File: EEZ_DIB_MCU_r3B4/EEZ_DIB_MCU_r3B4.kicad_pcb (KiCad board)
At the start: 4 copper layers, 139.5 x 70 mm, 119 parts, among them IC1 TPD4E001DRLR, IC11 TPS2051BDBVR, IC12 TPS61169DCKR, IC13 TPD4E001DRLR, IC14 TSC2007IPW, IC2 74AUP1G74DC.125, IC3 CD74HC4050PWR, IC5 LD1117ADT33TR, IC8 AT24C256C-SSHL-B, IC9 N.C., J1 5033981892, J2 67803-8020, J3 HR911130A, J4 Conn_01x22_Socket, Q1 N.C., Q2 2N7002, SW1 TL1100CF160Q, SW2 PEC16-2215F-S0024, U1 ICN6211, X1 DS1024-2*20R0, X2 DS1013-16SSIB1, X3 691322110005

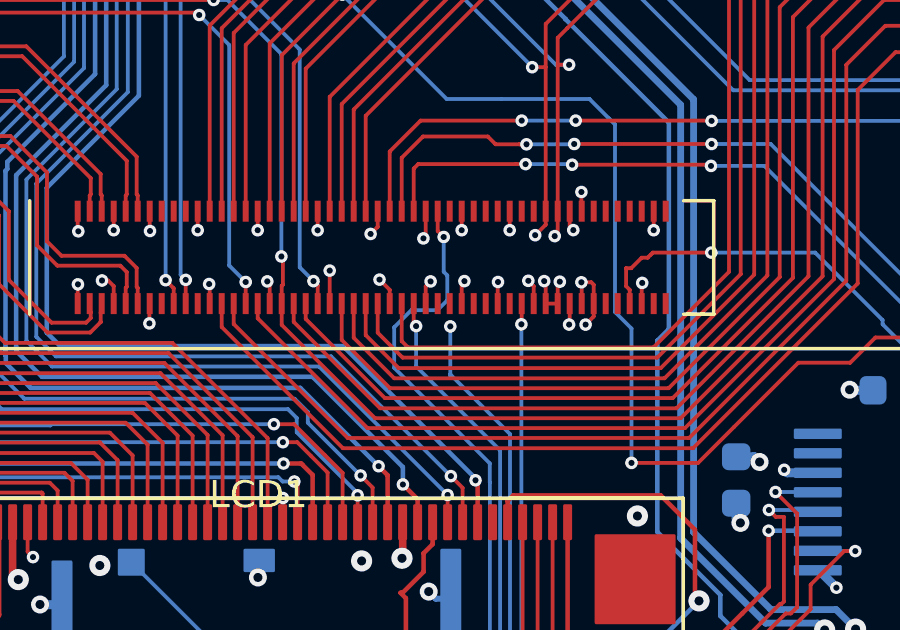
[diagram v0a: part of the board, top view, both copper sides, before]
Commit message: Routing
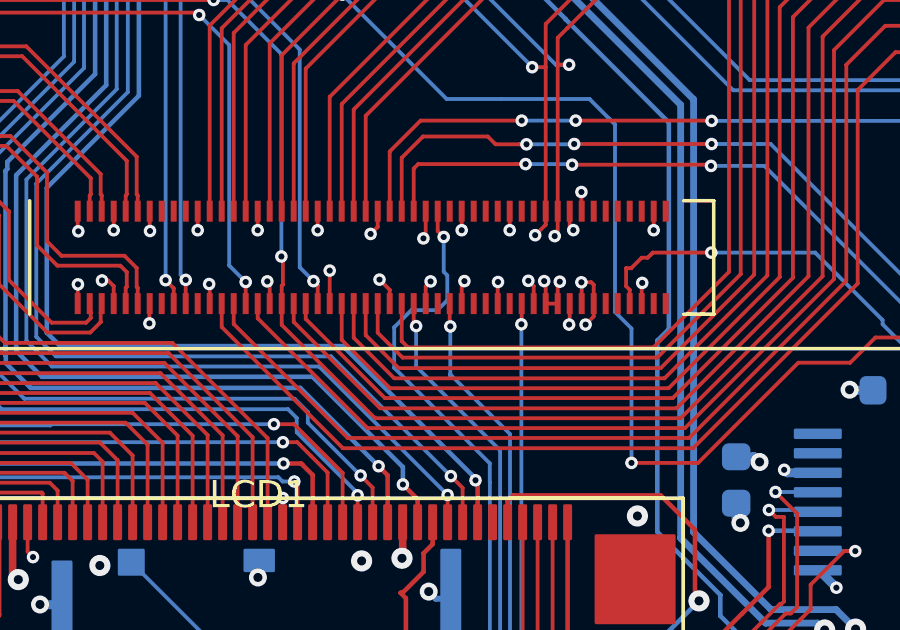
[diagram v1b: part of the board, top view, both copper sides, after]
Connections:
- Module1 pad 61: SDMMC1_D0 -> unconnected-(Module1A-SD_DAT3-Pad61)
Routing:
- net SDMMC1_D0: track 37.4 -> 38.2 mm
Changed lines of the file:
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@@
   (net 254 "unconnected-(J4-Pin_11-Pad11)")
   (net 255 "unconnected-(J4-Pin_12-Pad12)")
+  (net 256 "unconnected-(Module1A-SD_DAT3-Pad61)")
   (footprint "Resistor_SMD:R_0603_1608Metric" (layer "F.Cu")
     (at 127.4552 114.707 -90)
@@
     (pad "4" smd roundrect (at 0 -2.38 90) (size 5.8 6.2) (layers "F.Cu" "F.Paste" "F.Mask") (roundrect_rratio 0.00875862069)
       (net 117 "CM4_3.3V") (pinfunction "OUT") (pintype "passive") (solder_mask_margin 0.0635))
+    (model ":KICAD7_3DMODEL_DIR:Package_TO_SOT_SMD.3dshapes/TO-252-2.wrl"
+      (offset (xyz 0 0 0))
+      (scale (xyz 1 1 1))
+      (rotate (xyz 0 0 -90))
+    )
   )
   (footprint "EEZ_DIB_MCU_r3B4:DO214AA" (layer "F.Cu")
@@
       (net 1 "GND") (pinfunction "GND") (pintype "power_in"))
     (pad "61" smd rect (at -2 -19.3) (size 0.2 0.7) (layers "F.Cu" "F.Paste" "F.Mask")
-      (net 22 "SDMMC1_D0") (pinfunction "SD_DAT3") (pintype "passive"))
+      (net 256 "unconnected-(Module1A-SD_DAT3-Pad61)") (pinfunction "SD_DAT3") (pintype "passive+no_connect"))
     (pad "62" smd rect (at 1.08 -19.3) (size 0.2 0.7) (layers "F.Cu" "F.Paste" "F.Mask")
       (net 27 "SDMMC1_CMD") (pinfunction "SD_CMD") (pintype "passive"))
@@
     (pad "2" smd roundrect (at 1.9812 0 270) (size 2.8702 0.762) (layers "F.Cu" "F.Paste" "F.Mask") (roundrect_rratio 0.06666666667)
       (net 1 "GND") (pinfunction "-") (pintype "passive") (solder_mask_margin 0.0635))
+    (model ":KICAD7_3DMODEL_DIR:Capacitor_SMD.3dshapes/CP_Elec_5x4.4.step"
+      (offset (xyz 0 0 0))
+      (scale (xyz 1 1 1))
+      (rotate (xyz 0 0 0))
+    )
   )
   (footprint "EEZ_DIB_MCU_r3B4:EC1206" (layer "F.Cu")
@@
       (chamfer_ratio 0.2928932188) (chamfer top_left top_right bottom_left bottom_right)
       (net 51 "Net-(IC1-IO4)") (pinfunction "1") (pintype "passive") (solder_mask_margin 0.0635))
+    (model "${KIPRJMOD}/footprints/3D/138370836-659-691322110005/691322110005.stp"
+      (offset (xyz 0 -3.5 3.5))
+      (scale (xyz 1 1 1))
+      (rotate (xyz -90 0 0))
+    )
   )
   (footprint "EEZ_DIB_MCU_r3B4:DBV5" (layer "F.Cu")
@@
     (pad "2" smd roundrect (at 1.9812 0 180) (size 2.8702 0.762) (layers "F.Cu" "F.Paste" "F.Mask") (roundrect_rratio 0.06666666667)
       (net 1 "GND") (pinfunction "-") (pintype "passive") (solder_mask_margin 0.0635))
+    (model ":KICAD7_3DMODEL_DIR:Capacitor_SMD.3dshapes/CP_Elec_5x4.4.step"
+      (offset (xyz 0 0 0))
+      (scale (xyz 1 1 1))
+      (rotate (xyz 0 0 0))
+    )
   )
   (footprint "EEZ_DIB_MCU_r3B4:SOT23-BEC" (layer "F.Cu")
@@
     (pad "MP" smd rect (at -7.15 1.4) (size 1.8 2.2) (layers "F.Cu" "F.Paste" "F.Mask"))
     (pad "MP" smd rect (at 7.15 1.4) (size 1.8 2.2) (layers "F.Cu" "F.Paste" "F.Mask"))
-    (model "${KICAD6_3DMODEL_DIR}/Connector_FFC-FPC.3dshapes/Hirose_FH12-22S-0.5SH_1x22-1MP_P0.50mm_Horizontal.wrl"
+    (model "${KICAD7_3DMODEL_DIR}/Connector_FFC-FPC.3dshapes/Hirose_FH12-22S-0.5SH_1x22-1MP_P0.50mm_Horizontal.wrl"
       (offset (xyz 0 0 0))
       (scale (xyz 1 1 1))
       (rotate (xyz 0 0 0))
     )
+    (model ":KICAD7_3DMODEL_DIR:Connector_FFC-FPC.3dshapes/TE_2-84953-2_1x22-1MP_P1.0mm_Horizontal.wrl"
+      (offset (xyz 0 -0.5 0))
+      (scale (xyz 0.5 0.9 0.5))
+      (rotate (xyz 0 0 0))
+    )
   )
   (footprint "EEZ_DIB_MCU_r3B4:FPC_40" (layer "F.Cu")
@@
   (segment (start 105.1 104.34) (end 112.583333 111.823333) (width 0.127) (layer "B.Cu") (net 21))
   (segment (start 96.96 104.35) (end 98.54 104.35) (width 0.127) (layer "B.Cu") (net 21))
-  (segment (start 94.4 110.4) (end 94.42 110.42) (width 0.127) (layer "F.Cu") (net 22))
+  (segment (start 94.42 110.42) (end 94.4 110.4) (width 0.127) (layer "F.Cu") (net 22))
+  (segment (start 94.4 110.4) (end 94.4 109.66) (width 0.127) (layer "F.Cu") (net 22))
   (segment (start 89.77 126.11) (end 92.18 128.52) (width 0.127) (layer "F.Cu") (net 22))
   (segment (start 80.04 126.11) (end 89.77 126.11) (width 0.127) (layer "F.Cu") (net 22))
